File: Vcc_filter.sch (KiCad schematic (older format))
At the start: 15 parts

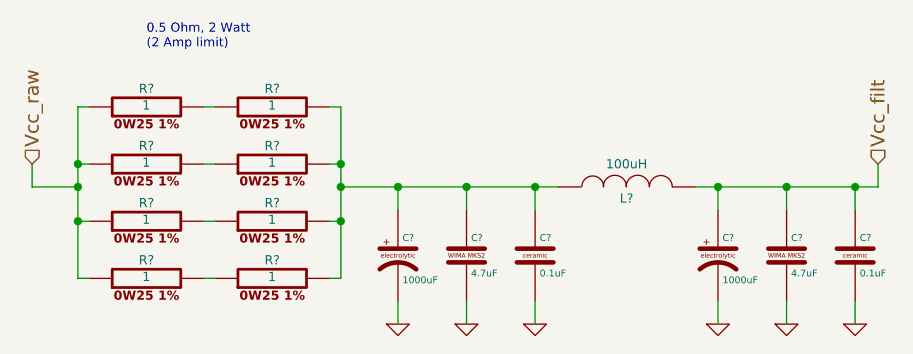
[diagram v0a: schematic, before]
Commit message: working on revamp of power supply.
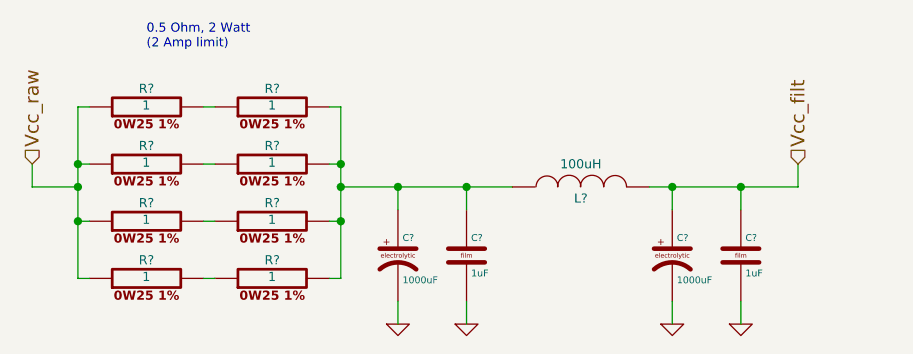
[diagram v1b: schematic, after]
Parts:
- removed C? (x2): 4.7uF, ~, symbol C_MKS2
- removed C? (x2): 0.1uF, ~, symbol C_CER
- added C? (x2): 1uF, ~, symbol C_FILM
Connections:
- net GND: now also C?.2, C?.2
- net Vcc_filt: now also C?.1
- net at C?.1, L?.1, R?.2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: now also C?.1
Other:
- moved on the sheet: C?, L?
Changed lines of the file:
@@
 EESchema Schematic File Version 2
+LIBS:OpAmpPassXsistorBenchSupply-cache
 LIBS:opamps_PL
+LIBS:opto_PL
+LIBS:regulators_PL
+LIBS:relays_PL
+LIBS:resistors_PL
+LIBS:switches_PL
 LIBS:transistors_PL
+LIBS:analog_ICs_PL
+LIBS:capacitors_PL
+LIBS:connectors_PL
 LIBS:diodes_PL
-LIBS:resistors_PL
-LIBS:capacitors_PL
-LIBS:regulators_PL
-LIBS:connectors_PL
+LIBS:displays_PL
+LIBS:LEDs_PL
+LIBS:microcontrollers_PL
+LIBS:mounting_holes_PL
 LIBS:power
 LIBS:device
@@
 $Descr A4 11693 8268
 encoding utf-8
-Sheet 3 9
+Sheet 3 5
 Title ""
 Date "4 jul 2014"
@@
 L INDUCTOR L?
 U 1 1 53375603
-P 5900 3700
-F 0 "L?" V 5850 3700 40  0000 C CNN
-F 1 "100uH" V 6000 3700 40  0000 C CNN
-F 2 "~" H 5900 3700 60  0000 C CNN
-F 3 "~" H 5900 3700 60  0000 C CNN
-	1    5900 3700
+P 5700 3700
+F 0 "L?" V 5650 3700 40  0000 C CNN
+F 1 "100uH" V 5800 3700 40  0000 C CNN
+F 2 "~" H 5700 3700 60  0000 C CNN
+F 3 "~" H 5700 3700 60  0000 C CNN
+	1    5700 3700
 	0    -1   -1   0
 $EndComp
@@
 L C_EL C?
 U 1 1 53375609
-P 6300 4000
-F 0 "C?" H 6320 4060 30  0000 L BNN
-F 1 "1000uF" H 6320 3910 30  0000 L TNN
-F 2 "~" H 6338 3850 30  0000 C CNN
-F 3 "~" H 6300 4000 60  0000 C CNN
-	1    6300 4000
-	1    0    0    -1
-$EndComp
-$Comp
-L C_MKS2 C?
-U 1 1 5337560F
-P 6600 4000
-F 0 "C?" H 6620 4060 30  0000 L BNN
-F 1 "4.7uF" H 6620 3940 30  0000 L TNN
-F 2 "~" H 6638 3850 30  0000 C CNN
-F 3 "~" H 6600 4000 60  0000 C CNN
-	1    6600 4000
-	1    0    0    -1
-$EndComp
-$Comp
-L C_CER C?
-U 1 1 53375615
-P 6900 4000
-F 0 "C?" H 6920 4060 30  0000 L BNN
-F 1 "0.1uF" H 6920 3940 30  0000 L TNN
-F 2 "~" H 6938 3850 30  0000 C CNN
-F 3 "~" H 6900 4000 60  0000 C CNN
-	1    6900 4000
-	1    0    0    -1
-$EndComp
-Wire Wire Line
-	6200 3700 7000 3700
-Wire Wire Line
-	7000 3700 7000 3600
-Wire Wire Line
-	6300 3800 6300 3700
-Connection ~ 6300 3700
-Wire Wire Line
-	6600 3800 6600 3700
-Connection ~ 6600 3700
-Wire Wire Line
-	6900 3800 6900 3700
-Connection ~ 6900 3700
+P 6100 4000
+F 0 "C?" H 6120 4060 30  0000 L BNN
+F 1 "1000uF" H 6120 3910 30  0000 L TNN
+F 2 "~" H 6138 3850 30  0000 C CNN
+F 3 "~" H 6100 4000 60  0000 C CNN
+	1    6100 4000
+	1    0    0    -1
+$EndComp
+Wire Wire Line
+	6000 3700 6100 3700
+Wire Wire Line
+	6100 3700 6400 3700
+Wire Wire Line
+	6400 3700 6650 3700
+Wire Wire Line
+	6650 3700 6650 3600
+Wire Wire Line
+	6100 3800 6100 3700
+Connection ~ 6100 3700
+Wire Wire Line
+	6400 3800 6400 3700
+Connection ~ 6400 3700
 $Comp
 L GND #PWR?
 U 1 1 53375623
-P 6300 4300
-F 0 "#PWR?" H 6300 4300 30  0001 C CNN
-F 1 "GND" H 6300 4230 30  0001 C CNN
-F 2 "" H 6300 4300 60  0000 C CNN
-F 3 "" H 6300 4300 60  0000 C CNN
-	1    6300 4300
+P 6100 4300
+F 0 "#PWR?" H 6100 4300 30  0001 C CNN
+F 1 "GND" H 6100 4230 30  0001 C CNN
+F 2 "" H 6100 4300 60  0000 C CNN
+F 3 "" H 6100 4300 60  0000 C CNN
+	1    6100 4300
 	1    0    0    -1
 $EndComp
@@
 L GND #PWR?
 U 1 1 53375629
-P 6600 4300
-F 0 "#PWR?" H 6600 4300 30  0001 C CNN
-F 1 "GND" H 6600 4230 30  0001 C CNN
-F 2 "" H 6600 4300 60  0000 C CNN
-F 3 "" H 6600 4300 60  0000 C CNN
-	1    6600 4300
-	1    0    0    -1
-$EndComp
-$Comp
-L GND #PWR?
-U 1 1 5337562F
-P 6900 4300
-F 0 "#PWR?" H 6900 4300 30  0001 C CNN
-F 1 "GND" H 6900 4230 30  0001 C CNN
-F 2 "" H 6900 4300 60  0000 C CNN
-F 3 "" H 6900 4300 60  0000 C CNN
-	1    6900 4300
-	1    0    0    -1
-$EndComp
-Wire Wire Line
-	6300 4200 6300 4300
-Wire Wire Line
-	6600 4200 6600 4300
-Wire Wire Line
-	6900 4200 6900 4300
+P 6400 4300
+F 0 "#PWR?" H 6400 4300 30  0001 C CNN
+F 1 "GND" H 6400 4230 30  0001 C CNN
+F 2 "" H 6400 4300 60  0000 C CNN
+F 3 "" H 6400 4300 60  0000 C CNN
+	1    6400 4300
+	1    0    0    -1
+$EndComp
+Wire Wire Line
+	6100 4200 6100 4300
+Wire Wire Line
+	6400 4200 6400 4300
 Wire Wire Line
 	4600 3350 4650 3350
 Wire Wire Line
-	4650 3350 4650 4100
+	4650 3350 4650 3600
+Wire Wire Line
+	4650 3600 4650 3700
+Wire Wire Line
+	4650 3700 4650 3850
+Wire Wire Line
+	4650 3850 4650 4100
 Wire Wire Line
 	4650 3850 4600 3850
@@
 Connection ~ 4650 3600
 Wire Wire Line
-	4650 3700 5600 3700
+	4650 3700 4900 3700
+Wire Wire Line
+	4900 3700 5200 3700
+Wire Wire Line
+	5200 3700 5400 3700
 Connection ~ 4650 3700
 Wire Wire Line
-	3500 3350 3500 4100
+	3500 3350 3500 3600
+Wire Wire Line
+	3500 3600 3500 3700
+Wire Wire Line
+	3500 3700 3500 3850
+Wire Wire Line
+	3500 3850 3500 4100
 Connection ~ 3500 3600
 Wire Wire Line
@@
 $EndComp
 $Comp
-L C_MKS2 C?
-U 1 1 53375655
-P 5200 4000
-F 0 "C?" H 5220 4060 30  0000 L BNN
-F 1 "4.7uF" H 5220 3940 30  0000 L TNN
-F 2 "~" H 5238 3850 30  0000 C CNN
-F 3 "~" H 5200 4000 60  0000 C CNN
-	1    5200 4000
-	1    0    0    -1
-$EndComp
-$Comp
-L C_CER C?
-U 1 1 5337565B
-P 5500 4000
-F 0 "C?" H 5520 4060 30  0000 L BNN
-F 1 "0.1uF" H 5520 3940 30  0000 L TNN
-F 2 "~" H 5538 3850 30  0000 C CNN
-F 3 "~" H 5500 4000 60  0000 C CNN
-	1    5500 4000
-	1    0    0    -1
-$EndComp
-$Comp
 L GND #PWR?
 U 1 1 53375661
@@
 	1    0    0    -1
 $EndComp
-$Comp
-L GND #PWR?
-U 1 1 5337566D
-P 5500 4300
-F 0 "#PWR?" H 5500 4300 30  0001 C CNN
-F 1 "GND" H 5500 4230 30  0001 C CNN
-F 2 "" H 5500 4300 60  0000 C CNN
-F 3 "" H 5500 4300 60  0000 C CNN
-	1    5500 4300
-	1    0    0    -1
-$EndComp
 Wire Wire Line
 	4900 4200 4900 4300
 Wire Wire Line
 	5200 4200 5200 4300
-Wire Wire Line
-	5500 4200 5500 4300
 Wire Wire Line
 	4900 3800 4900 3700
@@
 	5200 3800 5200 3700
 Connection ~ 5200 3700
-Wire Wire Line
-	5500 3800 5500 3700
-Connection ~ 5500 3700
 Text Notes 3800 3100 0    40   ~ 0
 0.5 Ohm, 2 Watt\n(2 Amp limit)
 Text HLabel 3300 3600 1    60   Input ~ 0
 Vcc_raw
-Text HLabel 7000 3600 1    60   Input ~ 0
+Text HLabel 6650 3600 1    60   Input ~ 0
 Vcc_filt
 $Comp
@@
 	0    -1   -1   0
 $EndComp
+$Comp
+L C_FILM C?
+U 1 1 53B62FA8
+P 5200 4000
+F 0 "C?" H 5220 4060 30  0000 L BNN
+F 1 "1uF" H 5220 3940 30  0000 L TNN
+F 2 "~" H 5238 3850 30  0000 C CNN
+F 3 "~" H 5200 4000 60  0000 C CNN
+	1    5200 4000
+	1    0    0    -1
+$EndComp
+$Comp
+L C_FILM C?
+U 1 1 53B62FBC
+P 6400 4000
+F 0 "C?" H 6420 4060 30  0000 L BNN
+F 1 "1uF" H 6420 3940 30  0000 L TNN
+F 2 "~" H 6438 3850 30  0000 C CNN
+F 3 "~" H 6400 4000 60  0000 C CNN
+	1    6400 4000
+	1    0    0    -1
+$EndComp
 $EndSCHEMATC
